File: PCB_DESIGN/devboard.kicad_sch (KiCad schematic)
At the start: 33 parts, among them J1 USB_C_Receptacle_USB2.0_14P, J2 Conn_01x20, J3 Conn_01x20, J4 Conn_01x03, SW1 SW_Push, U1 RP2040, U2 NCP1117-3.3_SOT223, U3 W25Q128JVS, Y1 12 MHz

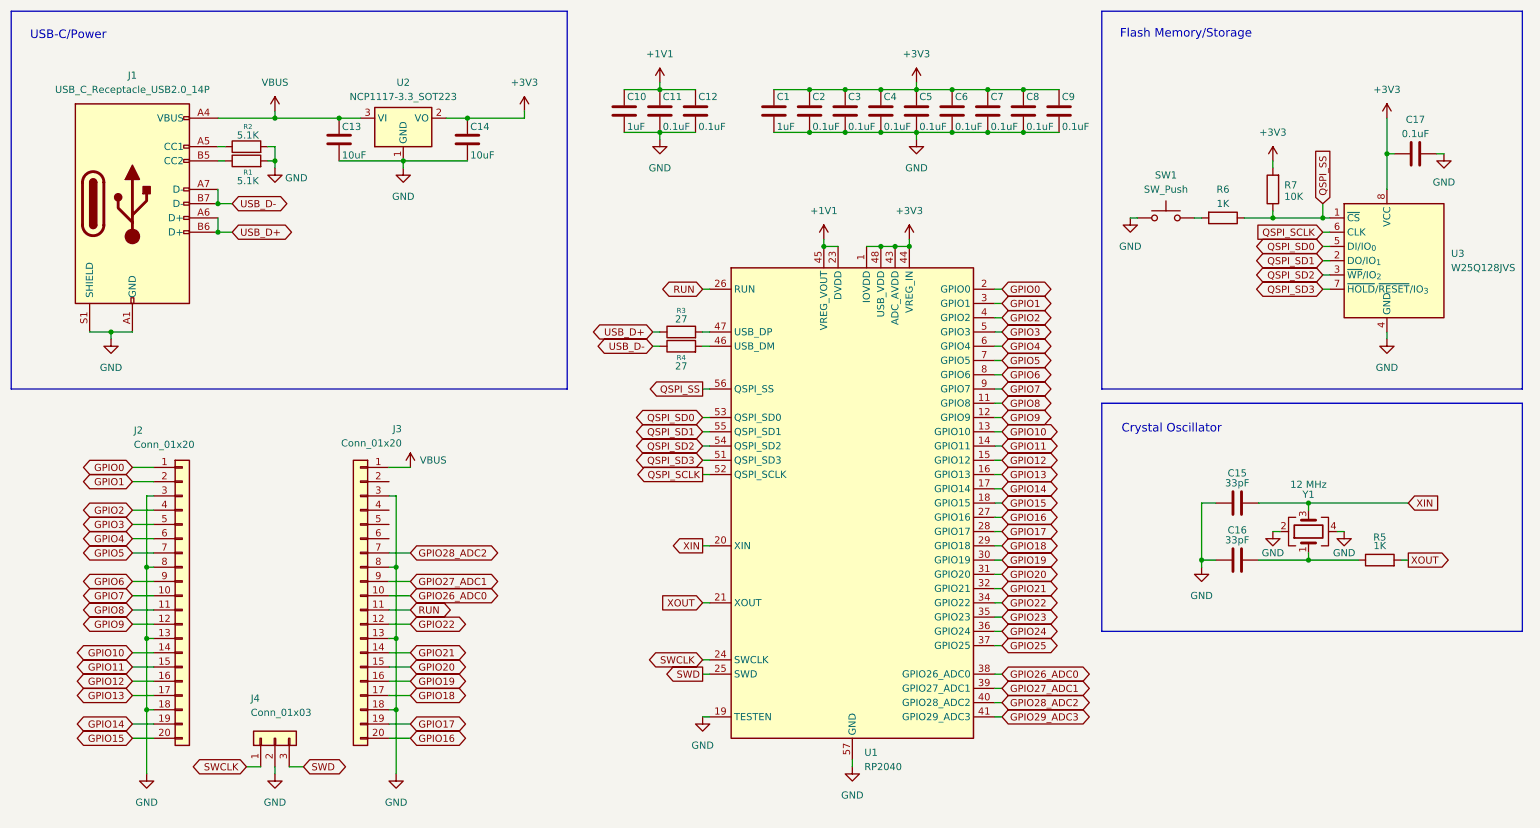
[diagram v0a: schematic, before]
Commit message: finishing the schematic refined
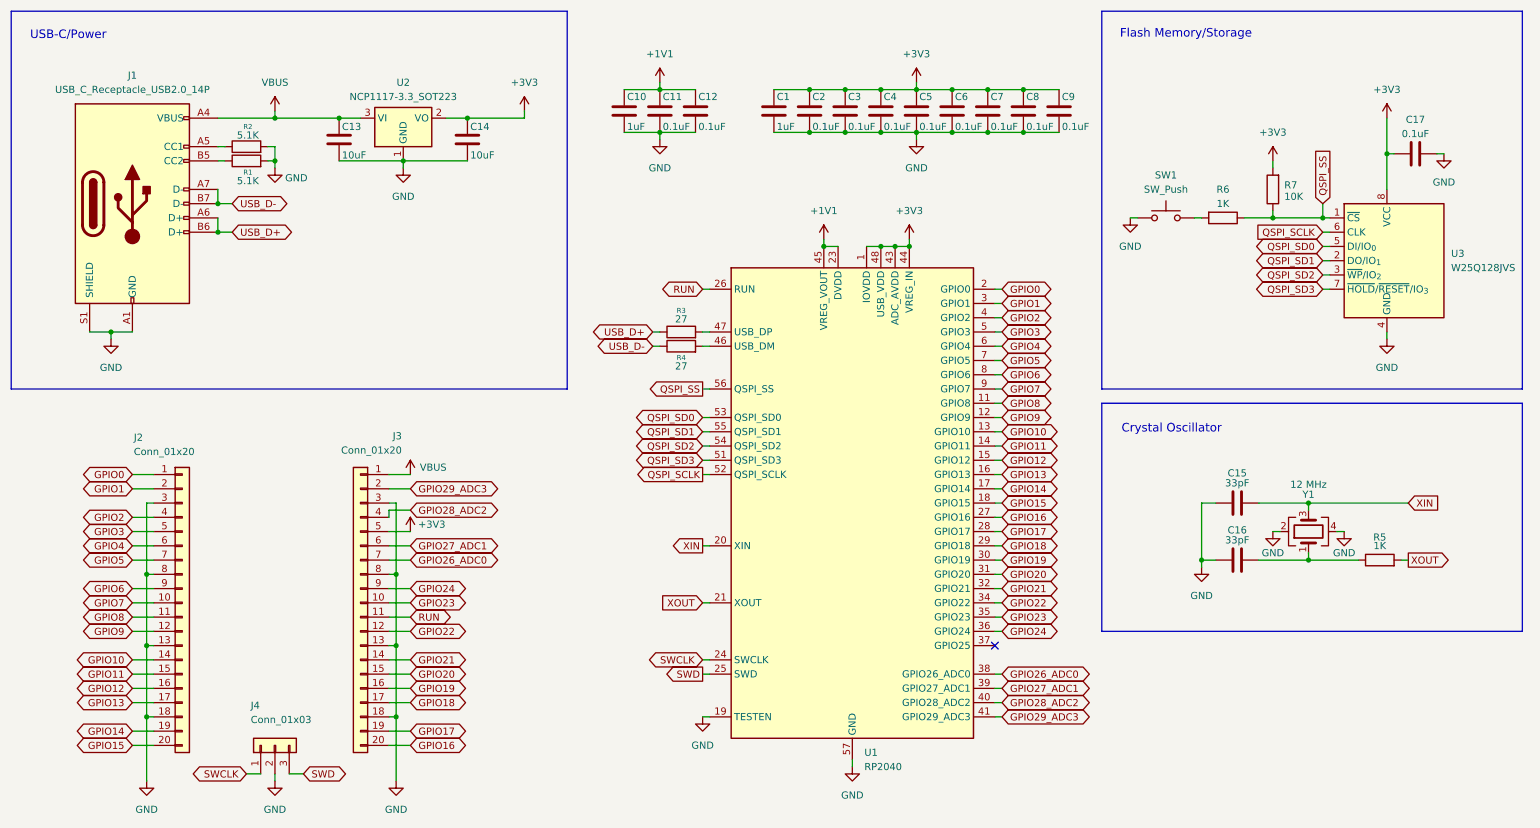
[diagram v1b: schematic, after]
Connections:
- net +3V3: now also J3.5 (Pin_5)
- net GPIO23: now also J3.10 (Pin_10)
- net GPIO24: now also J3.9 (Pin_9)
- net GPIO26_ADC0: now also J3.7 (Pin_7); no longer J3.10 (Pin_10)
- net GPIO27_ADC1: now also J3.6 (Pin_6); no longer J3.9 (Pin_9)
- net GPIO28_ADC2: now also J3.4 (Pin_4); no longer J3.7 (Pin_7)
- net GPIO29_ADC3: now also J3.2 (Pin_2)
- net GPIO25: no longer names the net of U1.37 (GPIO25)
- no-connect marks 0 -> 1
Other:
- moved on the sheet: J2, J3, J4
